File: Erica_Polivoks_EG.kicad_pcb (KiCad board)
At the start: 2 copper layers, 40.3 x 106 mm, 92 parts, among them J1 GATE IN, J2 INV EG OUT, J3 Eurorack_Power_10pin_Unshroud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, J4 GATE D.OUT, J5 EG OUT, Q1 4, Q2 4, Q3 4, Q4 4, Q5 4, Q6 4, Q7 6, Q8 6, Q9 6, U1 TL074

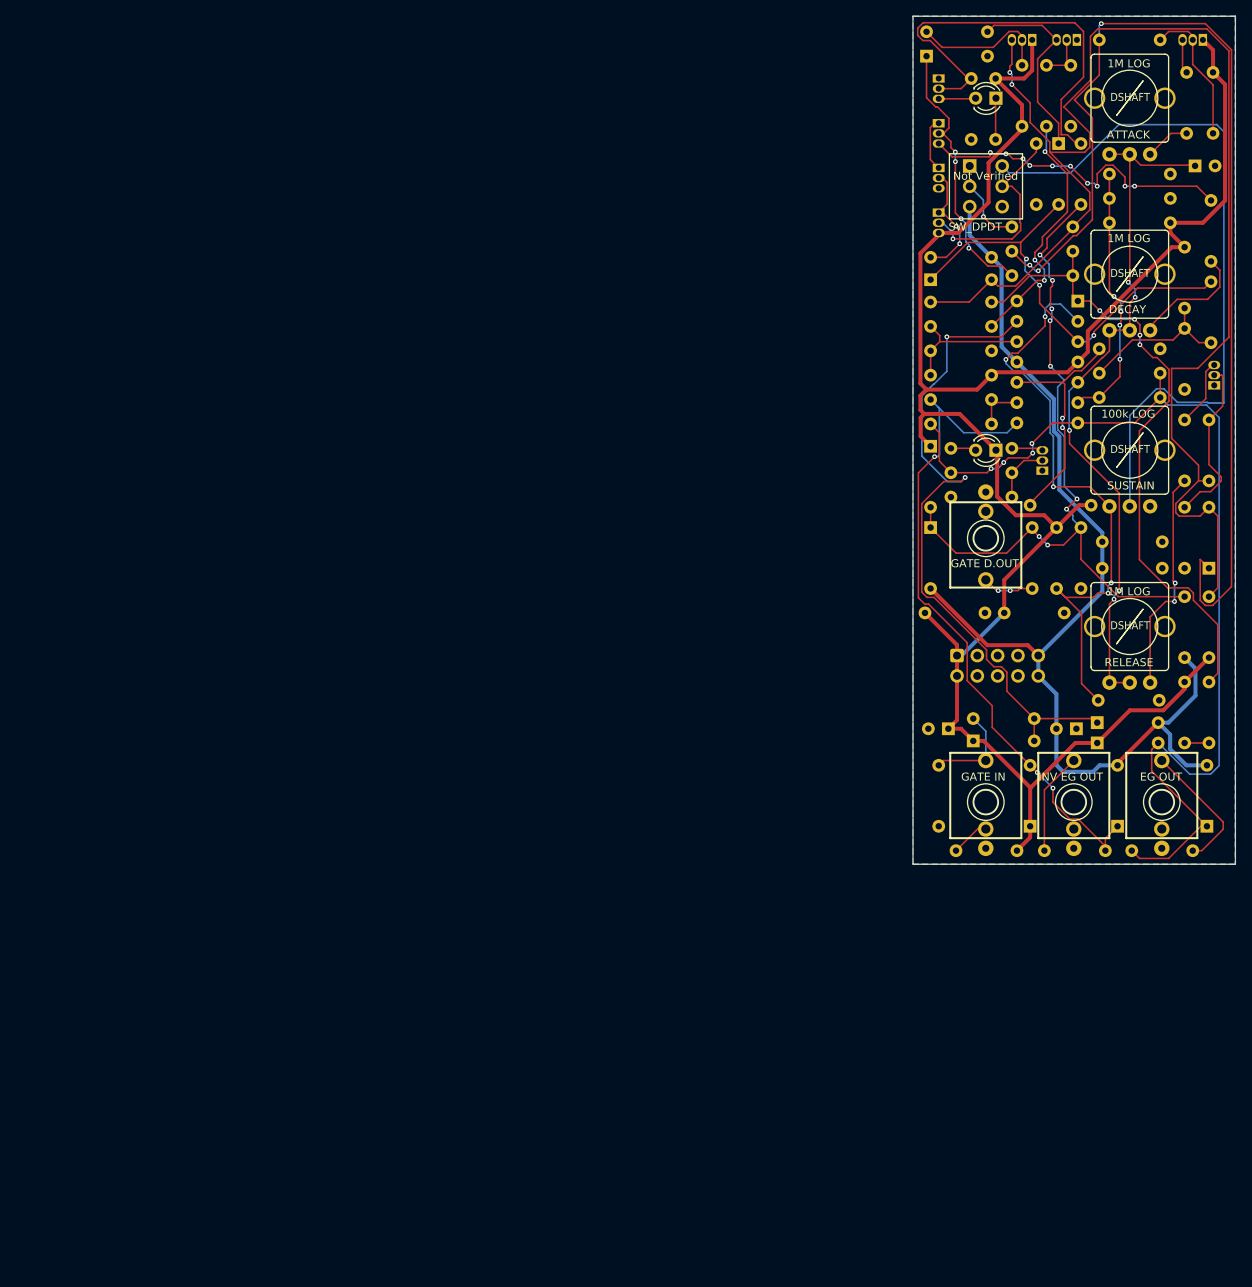
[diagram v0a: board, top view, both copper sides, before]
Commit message: almost ready to go
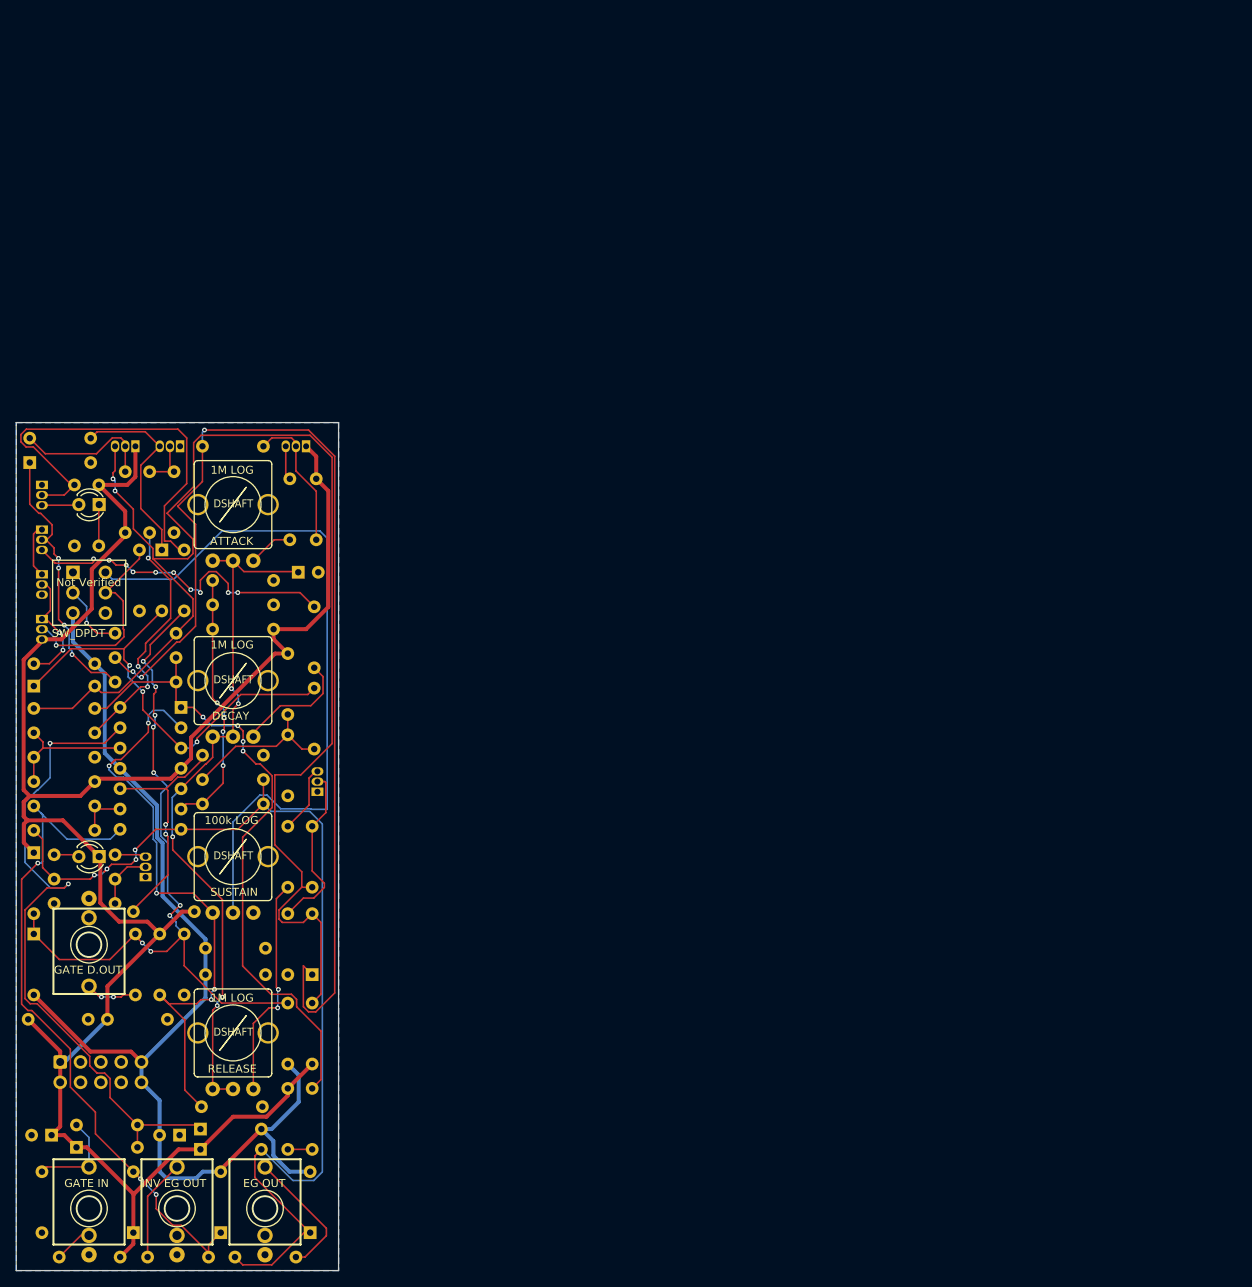
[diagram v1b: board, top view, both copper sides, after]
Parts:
- moved C1 123.1 mm to (79.6, 146.9)
- moved C2 123.1 mm to (82.5, 161.4)
- moved C3 123.1 mm to (89.5, 146.9)
- moved C7 123.1 mm to (113.3, 91.0)
- moved D1 123.1 mm to (101.1, 160.6)
- moved D11 123.1 mm to (87.2, 82.5)
- moved D12 123.1 mm to (80.3, 136.2)
- moved D13 123.1 mm to (80.3, 126.1)
- moved D15 123.1 mm to (101.1, 163.1)
- moved D18 123.1 mm to (87.2, 126.5)
- moved D2 123.1 mm to (85.6, 162.9)
- moved D3 123.1 mm to (96.3, 88.2)
- moved D4 123.1 mm to (115.1, 141.3)
- moved D5 123.1 mm to (80.3, 105.2)
- moved D8 123.1 mm to (92.7, 173.6)
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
